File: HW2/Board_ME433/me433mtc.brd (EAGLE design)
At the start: 50 x 50 mm, 22 parts, among them IC1 PIC32MX250F128B, IC2 MCP1702, J1 USBMINIB-MB-H, SW1 SLIDE, Y1 8MHz

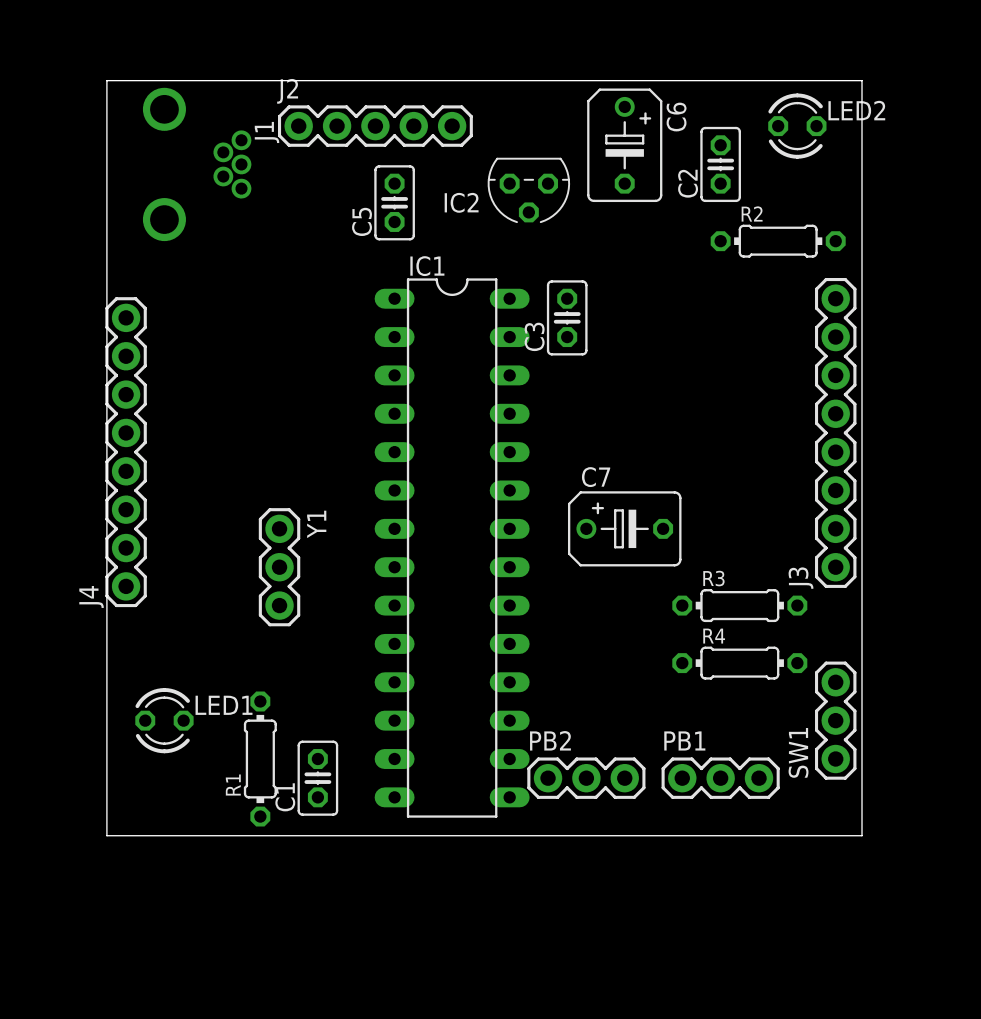
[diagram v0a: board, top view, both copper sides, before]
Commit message: finished board
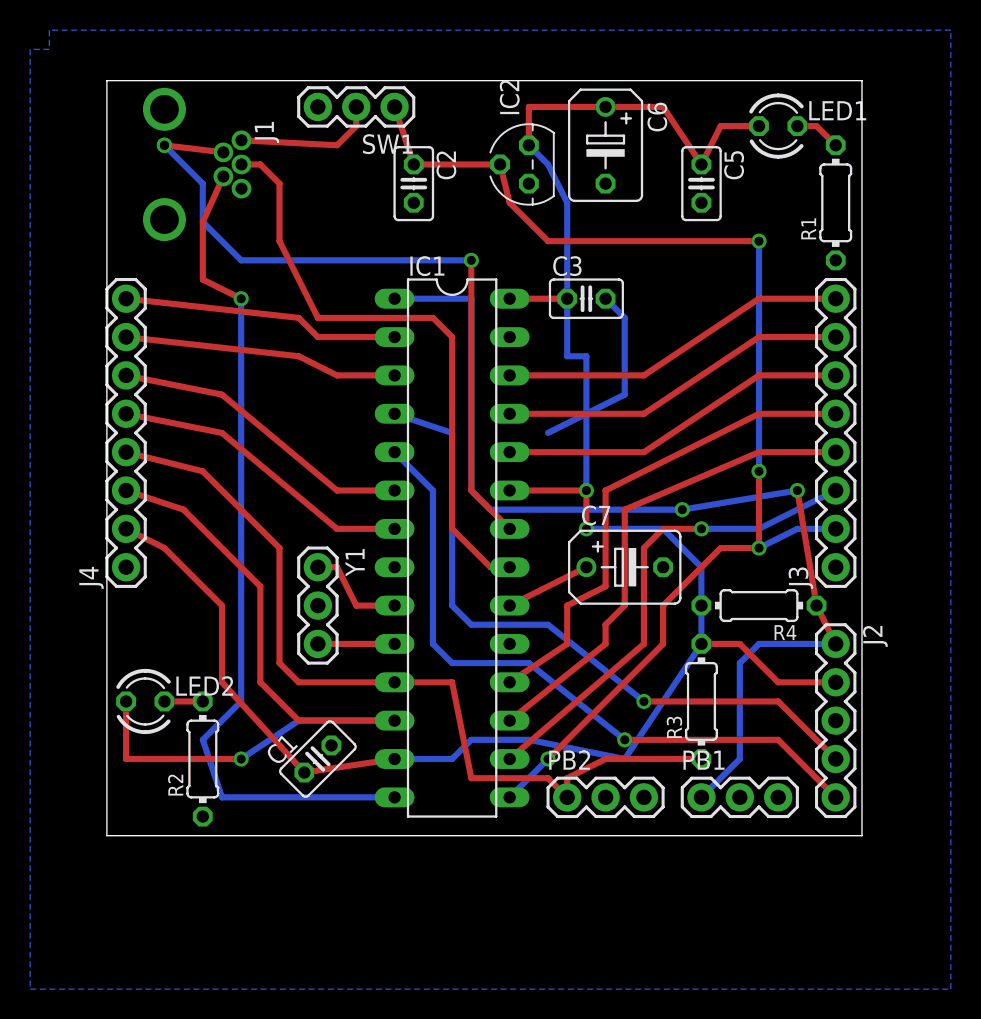
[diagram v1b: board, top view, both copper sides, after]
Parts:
- moved LED2 57.6 mm to (2.54, 8.89)
- moved LED1 56.6 mm to (44.5, 47.0)
- moved R1 53.0 mm to (48.3, 41.9)
- moved SW1 52.1 mm to (19.1, 48.3), turned to 180 degrees
- moved R2 51.3 mm to (6.35, 5.08), turned to 90 degrees
- moved J2 49.4 mm to (48.3, 12.7), turned to 270 degrees
- moved C2 20.4 mm to (20.3, 43.2), turned to 270 degrees
- moved C5 20.4 mm to (39.4, 43.2), turned to 270 degrees
- moved R3 6.84 mm to (39.4, 8.89), turned to 90 degrees
- moved R4 4.02 mm to (43.2, 15.2), turned to 180 degrees
- moved Y1 3.59 mm to (14.0, 17.8)
- moved C7 2.54 mm to (34.3, 17.8)
- moved C3 1.80 mm to (31.8, 35.6), turned to 0 degrees
- moved PB2 1.80 mm to (30.5, 2.54)
- moved PB1 1.80 mm to (39.4, 2.54)
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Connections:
- removed net N$16: C3.1, IC1.13
- net +3V3: now also C3.1, IC1.13
- net B4/USER: now also R3.1
- net MCLR: now also R4.1
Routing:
- net +3V3: track 0.00 -> 134.0 mm, vias 0 -> 2
- net +5V: track 0.00 -> 80.4 mm, vias 0 -> 4
- net MCLR: track 0.00 -> 67.4 mm, vias 0 -> 2
- net B4/USER: track 0.00 -> 55.8 mm
- net USBID: track 0.00 -> 55.7 mm, vias 0 -> 1
- net A4/LED: track 0.00 -> 49.9 mm, vias 0 -> 1
- net D-: track 0.00 -> 47.7 mm, vias 0 -> 2
- net PGD: track 0.00 -> 44.7 mm, vias 0 -> 1
- net PGC: track 0.00 -> 44.3 mm, vias 0 -> 1
- net D+: track 0.00 -> 39.5 mm
- net B9: track 0.00 -> 32.7 mm
- net B8: track 0.00 -> 32.3 mm
- net B7: track 0.00 -> 31.9 mm, vias 0 -> 1
- net B15: track 0.00 -> 23.1 mm
- net B14: track 0.00 -> 23.1 mm
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- added copper zone on layer 16, net GND
